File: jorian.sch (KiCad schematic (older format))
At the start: 101 parts, among them J1 USB-C, J2 USB-C, J3 MicroUSB, J4 MicroUSB, J5 MJ-4PP-9, Q1 AO3407, SW1 MSK-12C02, U1 E73-2G4M08S1C-52840, U2 E73-2G4M08S1C-52840, U3 MCP73831, X1 10uH

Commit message: updated files
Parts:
- removed H1: Battery Pad, kbd:battery_pad, symbol Mechanical:MountingHole_Pad
- removed JP1: +, kbd:jumper, symbol Device:Jumper_NO_Small
- removed JP10: -, kbd:jumper, symbol Device:Jumper_NO_Small
- removed JP16, JP25, JP26, JP27, JP28, JP29, JP30, JP31: (no value), kbd:jumper, symbol Device:Jumper_NO_Small
- removed OLED2: I2C_conn, kbd:connector_i2c, symbol Connector_Generic:Conn_01x04
- added Q2: SI2306, Package_TO_SOT_SMD:SOT-23, symbol Transistor_FET:BS870
- added R3: 10K, Resistor_SMD:R_0603_1608Metric, symbol Device:R
- JP11: symbol Connector_Generic:Conn_01x04 -> Connector_Generic:Conn_01x02
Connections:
- net labels added: LED_GND
- net labels removed: PGND
- wire segments 334 -> 317
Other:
- note added: "Power Control\nNormally On\nLow - Off\n"
- moved on the sheet: J5, U1, U2, X1

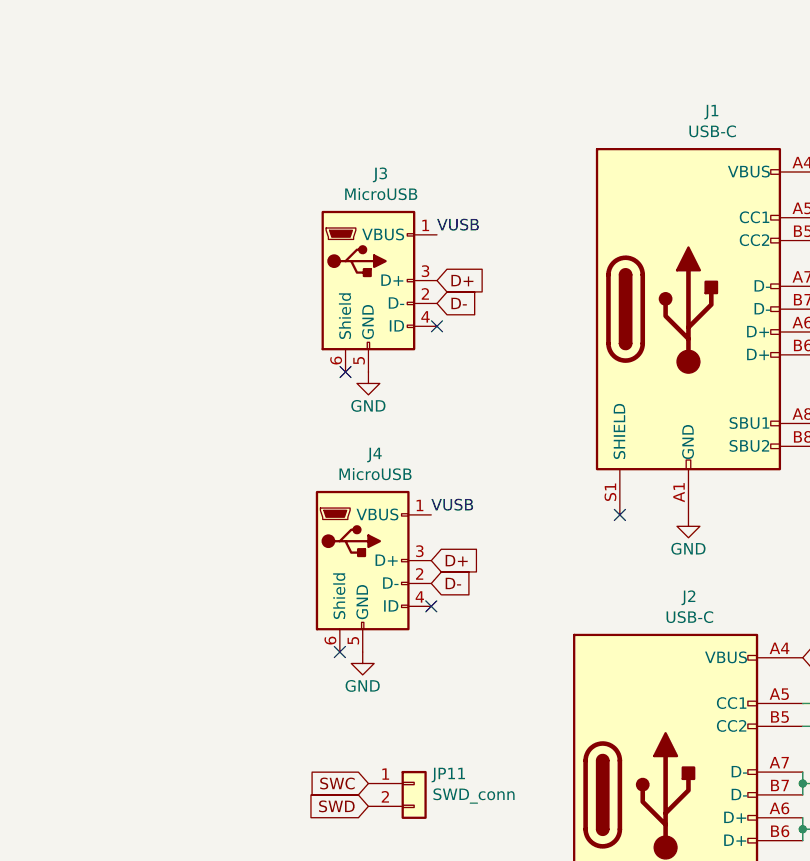
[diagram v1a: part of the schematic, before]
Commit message: updated files
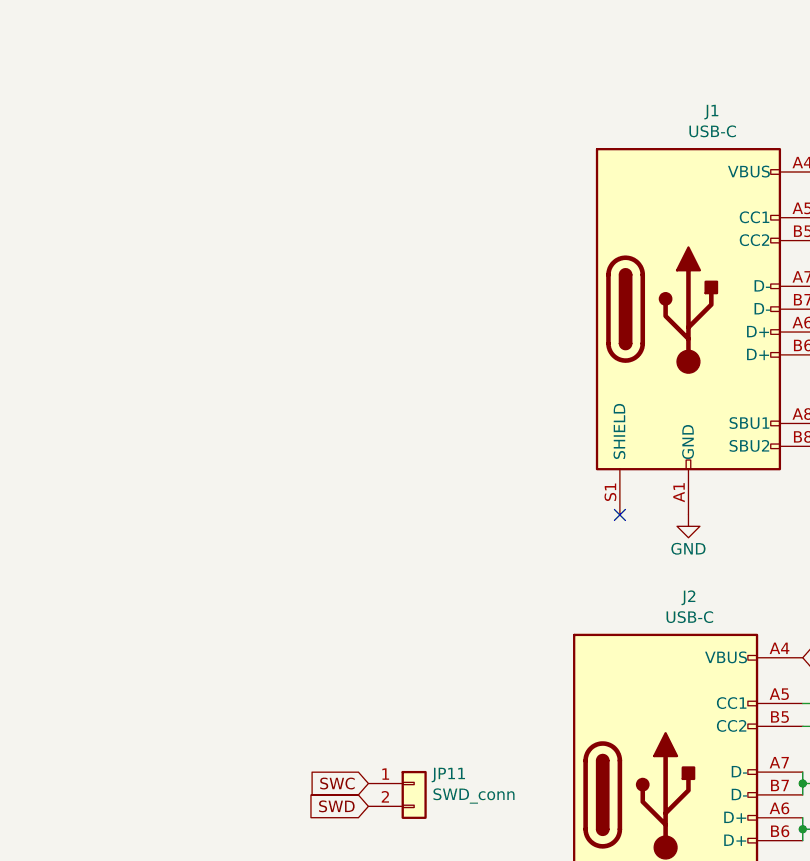
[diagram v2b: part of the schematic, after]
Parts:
- removed J3, J4: MicroUSB, kbd:usb_micro_custom, symbol Connector:USB_B_Micro
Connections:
- no-connect marks 18 -> 14
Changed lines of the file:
@@
 	8000 9300 8500 9300
-$Comp
-L Connector:USB_B_Micro J3
-U 1 1 5DDAA442
-P 13125 5500
-F 0 "J3" H 13180 5967 50  0000 C CNN
-F 1 "MicroUSB" H 13180 5876 50  0000 C CNN
-F 2 "kbd:usb_micro_custom" H 13275 5450 50  0001 C CNN
-F 3 "~" H 13275 5450 50  0001 C CNN
-	1    13125 5500
-	1    0    0    -1
-$EndComp
-Text Label 13425 5300 0    50   ~ 0
-VUSB
-NoConn ~ 13025 5900
 $Comp
 L power:GND #PWR0108
@@
 Wire Wire Line
 	15125 5525 15125 5575
-NoConn ~ 13000 7125
-NoConn ~ 13400 6925
 NoConn ~ 14225 6525
 NoConn ~ 15125 6225
@@
 NoConn ~ 15125 5325
 NoConn ~ 15125 5225
-Text Label 13400 6525 0    50   ~ 0
-VUSB
-$Comp
-L Connector:USB_B_Micro J4
-U 1 1 5DDAA45A
-P 13100 6725
-F 0 "J4" H 13155 7192 50  0000 C CNN
-F 1 "MicroUSB" H 13155 7101 50  0000 C CNN
-F 2 "kbd:usb_micro_custom" H 13250 6675 50  0001 C CNN
-F 3 "~" H 13250 6675 50  0001 C CNN
-	1    13100 6725
-	1    0    0    -1
-$EndComp
 $Comp
 L jorian-rescue:USB_C_Receptacle_USB2.0-Connector J1
@@
 	1    0    0    -1
 $EndComp
-NoConn ~ 13425 5700
-$Comp
-L power:GND #PWR0109
-U 1 1 5DDAA46D
-P 13125 5900
-F 0 "#PWR0109" H 13125 5650 50  0001 C CNN
-F 1 "GND" H 13125 5750 50  0000 C CNN
-F 2 "" H 13125 5900 50  0001 C CNN
-F 3 "" H 13125 5900 50  0001 C CNN
-	1    13125 5900
-	-1   0    0    -1
-$EndComp
-$Comp
-L power:GND #PWR0112
-U 1 1 5DDAA473
-P 13100 7125
-F 0 "#PWR0112" H 13100 6875 50  0001 C CNN
-F 1 "GND" H 13100 6975 50  0000 C CNN
-F 2 "" H 13100 7125 50  0001 C CNN
-F 3 "" H 13100 7125 50  0001 C CNN
-	1    13100 7125
-	-1   0    0    -1
-$EndComp
 Text GLabel 15225 5575 2    50   Input ~ 0
 D-
@@
 Wire Wire Line
 	15125 5775 15225 5775
-Text GLabel 13425 5500 2    50   Input ~ 0
-D+
-Text GLabel 13425 5600 2    50   Input ~ 0
-D-
-Text GLabel 13400 6825 2    50   Input ~ 0
-D-
-Text GLabel 13400 6725 2    50   Input ~ 0
-D+
 Text GLabel 15125 5025 2    50   Input ~ 0
 VUSB

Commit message: updated files
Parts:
- removed JP18: LIPO+, kbd:jumper, symbol Device:Jumper_NO_Small
- removed JP19: LIPO-, kbd:jumper, symbol Device:Jumper_NO_Small
- removed JP20: BAT+, kbd:jumper, symbol Device:Jumper_NO_Small
- removed JP21: BAT-, kbd:jumper, symbol Device:Jumper_NO_Small
- added Q3: AO3407, Package_TO_SOT_SMD:SOT-23, symbol Transistor_FET:BSS83P
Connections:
- net labels added: LED_VCC
- net labels removed: LED_GND, LIPO+, LIPO-
- wire segments 317 -> 320
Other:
- moved on the sheet: BT1, C1, C2, C3, D1, D2, JP11, JP2, JP3, JP4, JP5, JP6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

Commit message: updated files
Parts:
- removed J2: USB-C, kbd:usb_type_c, symbol jorian-rescue:USB_C_Receptacle_USB2.0-Connector
- removed U2: E73-2G4M08S1C-52840, kbd:E73-2G4M08S1C-52840, symbol jorian-rescue:E73-2G4M08S1C-52840
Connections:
- net labels added: CC1, CC2
- wire segments 320 -> 303
- no-connect marks 14 -> 8
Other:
- moved on the sheet: R1, R2

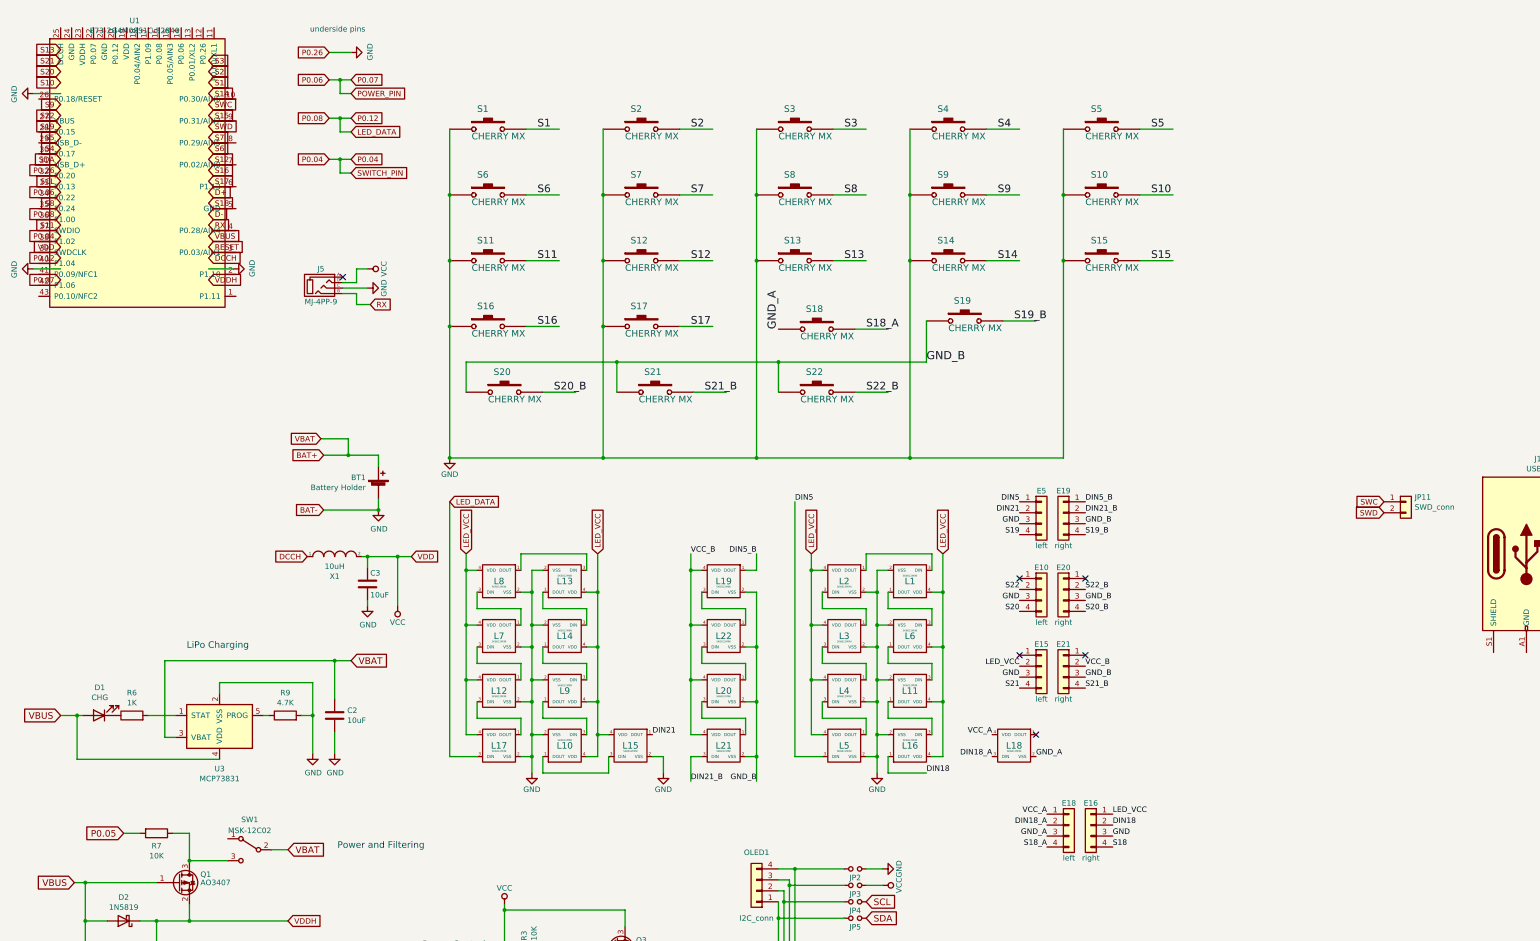
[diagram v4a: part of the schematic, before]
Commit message: autorouted
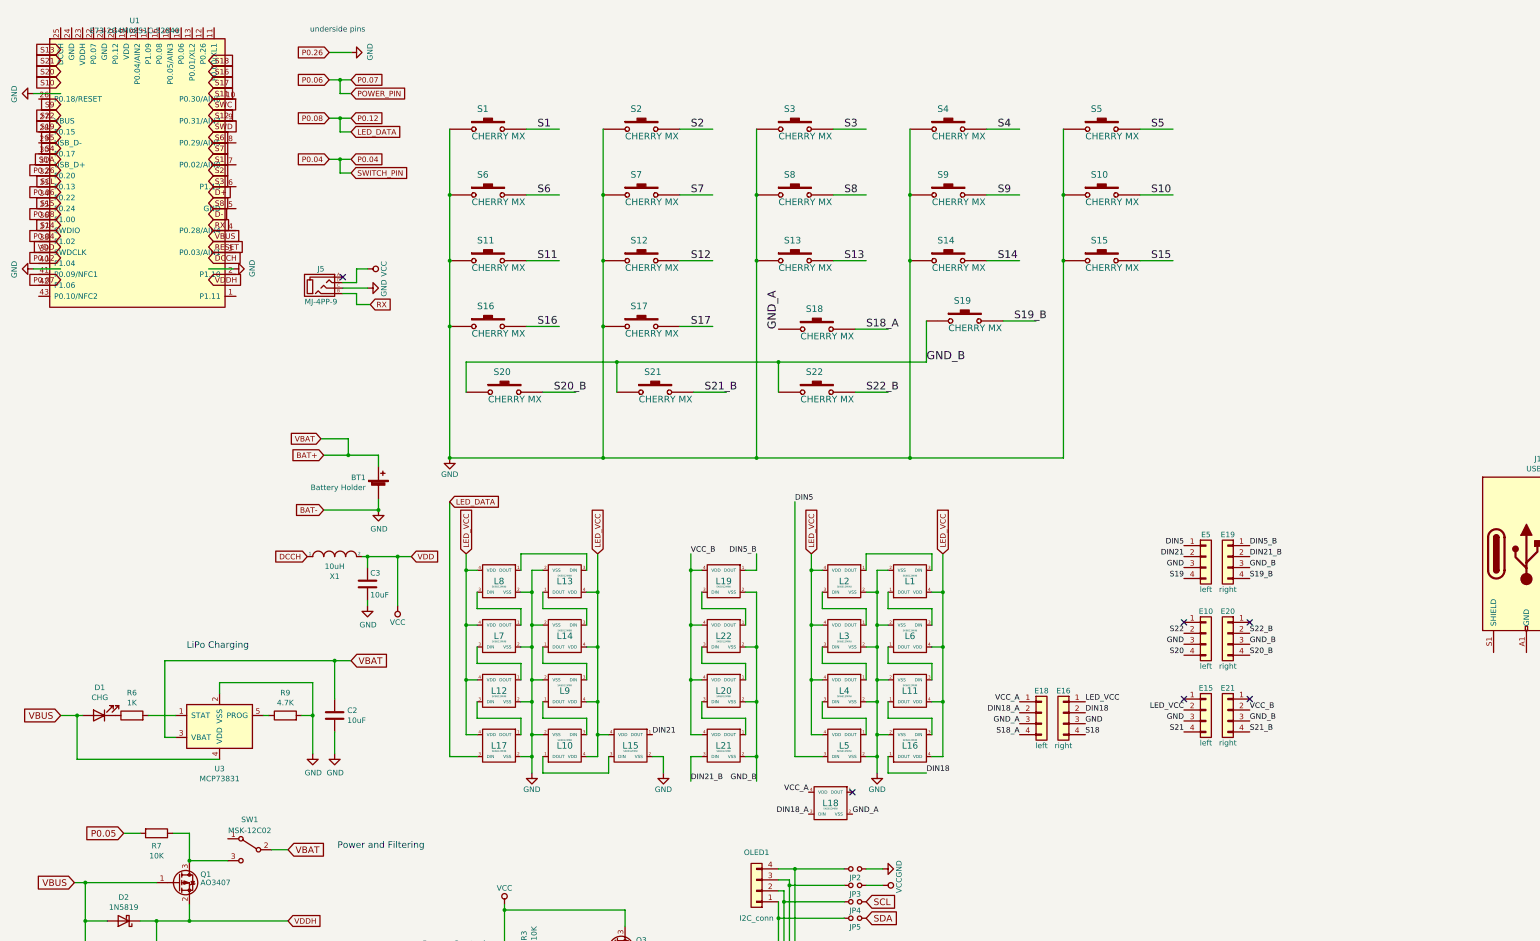
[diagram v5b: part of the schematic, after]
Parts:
- removed JP11: SWD_conn, kbd:connector_swd, symbol Connector_Generic:Conn_01x02
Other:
- moved on the sheet: E10, E15, E16, E18, E19, E20, E21, E5, L18
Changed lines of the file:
@@
 L Connector_Generic:Conn_01x04 E16
 U 1 1 5C28A7CD
-P 10550 8100
-F 0 "E16" H 10550 8300 50  0000 C CNN
-F 1 "right" H 10550 7800 50  0000 C CNN
-F 2 "kbd:edge_conn" H 10550 8100 50  0001 C CNN
-F 3 "" H 10550 8100 50  0001 C CNN
-	1    10550 8100
+P 10300 7075
+F 0 "E16" H 10300 7275 50  0000 C CNN
+F 1 "right" H 10300 6775 50  0000 C CNN
+F 2 "kbd:edge_conn" H 10300 7075 50  0001 C CNN
+F 3 "" H 10300 7075 50  0001 C CNN
+	1    10300 7075
 	-1   0    0    -1
 $EndComp
@@
 L Connector_Generic:Conn_01x04 E18
 U 1 1 5C28AA80
-P 10350 8100
-F 0 "E18" H 10350 8300 50  0000 C CNN
-F 1 "left" H 10350 7800 50  0000 C CNN
-F 2 "kbd:edge_conn" H 10350 8100 50  0001 C CNN
-F 3 "" H 10350 8100 50  0001 C CNN
-	1    10350 8100
-	1    0    0    -1
-$EndComp
-Text Label 10750 8200 0    50   ~ 0
+P 10100 7075
+F 0 "E18" H 10100 7275 50  0000 C CNN
+F 1 "left" H 10100 6775 50  0000 C CNN
+F 2 "kbd:edge_conn" H 10100 7075 50  0001 C CNN
+F 3 "" H 10100 7075 50  0001 C CNN
+	1    10100 7075
+	1    0    0    -1
+$EndComp
+Text Label 10500 7175 0    50   ~ 0
 GND
-Text Label 10750 8300 0    50   ~ 0
+Text Label 10500 7275 0    50   ~ 0
 S18
-Text Label 10750 8000 0    50   ~ 0
+Text Label 10500 6975 0    50   ~ 0
 LED_VCC
 $Comp
 L Connector_Generic:Conn_01x04 E19
 U 1 1 5C6E087C
-P 10300 5250
-F 0 "E19" H 10300 5450 50  0000 C CNN
-F 1 "right" H 10300 4950 50  0000 C CNN
-F 2 "kbd:edge_conn" H 10300 5250 50  0001 C CNN
-F 3 "" H 10300 5250 50  0001 C CNN
-	1    10300 5250
+P 11800 5650
+F 0 "E19" H 11800 5850 50  0000 C CNN
+F 1 "right" H 11800 5350 50  0000 C CNN
+F 2 "kbd:edge_conn" H 11800 5650 50  0001 C CNN
+F 3 "" H 11800 5650 50  0001 C CNN
+	1    11800 5650
 	-1   0    0    -1
 $EndComp
@@
 L Connector_Generic:Conn_01x04 E5
 U 1 1 5C6E0883
-P 10100 5250
-F 0 "E5" H 10100 5450 50  0000 C CNN
-F 1 "left" H 10100 4950 50  0000 C CNN
-F 2 "kbd:edge_conn" H 10100 5250 50  0001 C CNN
-F 3 "" H 10100 5250 50  0001 C CNN
-	1    10100 5250
-	1    0    0    -1
-$EndComp
-Text Label 9900 5450 2    50   ~ 0
+P 11600 5650
+F 0 "E5" H 11600 5850 50  0000 C CNN
+F 1 "left" H 11600 5350 50  0000 C CNN
+F 2 "kbd:edge_conn" H 11600 5650 50  0001 C CNN
+F 3 "" H 11600 5650 50  0001 C CNN
+	1    11600 5650
+	1    0    0    -1
+$EndComp
+Text Label 11400 5850 2    50   ~ 0
 S19
-Text Label 9900 6150 2    50   ~ 0
+Text Label 11400 6550 2    50   ~ 0
 S20
 $Comp
 L Connector_Generic:Conn_01x04 E21
 U 1 1 5C6F2906
-P 10300 6650
-F 0 "E21" H 10300 6850 50  0000 C CNN
-F 1 "right" H 10300 6350 50  0000 C CNN
-F 2 "kbd:edge_conn" H 10300 6650 50  0001 C CNN
-F 3 "" H 10300 6650 50  0001 C CNN
-	1    10300 6650
+P 11800 7050
+F 0 "E21" H 11800 7250 50  0000 C CNN
+F 1 "right" H 11800 6750 50  0000 C CNN
+F 2 "kbd:edge_conn" H 11800 7050 50  0001 C CNN
+F 3 "" H 11800 7050 50  0001 C CNN
+	1    11800 7050
 	-1   0    0    -1
 $EndComp
@@
 L Connector_Generic:Conn_01x04 E15
 U 1 1 5C6F290D
-P 10100 6650
-F 0 "E15" H 10100 6850 50  0000 C CNN
-F 1 "left" H 10100 6350 50  0000 C CNN
-F 2 "kbd:edge_conn" H 10100 6650 50  0001 C CNN
-F 3 "" H 10100 6650 50  0001 C CNN
-	1    10100 6650
-	1    0    0    -1
-$EndComp
-Text Label 9900 5950 2    50   ~ 0
+P 11600 7050
+F 0 "E15" H 11600 7250 50  0000 C CNN
+F 1 "left" H 11600 6750 50  0000 C CNN
+F 2 "kbd:edge_conn" H 11600 7050 50  0001 C CNN
+F 3 "" H 11600 7050 50  0001 C CNN
+	1    11600 7050
+	1    0    0    -1
+$EndComp
+Text Label 11400 6350 2    50   ~ 0
 S22
-Text Label 10750 8100 0    50   ~ 0
+Text Label 10500 7075 0    50   ~ 0
 DIN18
-Text Label 10150 8300 2    50   ~ 0
+Text Label 9900 7275 2    50   ~ 0
 S18_A
-Text Label 10150 8200 2    50   ~ 0
+Text Label 9900 7175 2    50   ~ 0
 GND_A
-Text Label 10150 8000 2    50   ~ 0
+Text Label 9900 6975 2    50   ~ 0
 VCC_A
-Text Label 10150 8100 2    50   ~ 0
+Text Label 9900 7075 2    50   ~ 0
 DIN18_A
-Text Label 10500 5450 0    50   ~ 0
+Text Label 12000 5850 0    50   ~ 0
 S19_B
-Text Label 10500 6150 0    50   ~ 0
+Text Label 12000 6550 0    50   ~ 0
 S20_B
-Text Label 10500 6850 0    50   ~ 0
+Text Label 12000 7250 0    50   ~ 0
 S21_B
-Text Label 10500 5950 0    50   ~ 0
+Text Label 12000 6350 0    50   ~ 0
 S22_B
-Text Label 10500 6650 0    50   ~ 0
+Text Label 12000 7050 0    50   ~ 0
 VCC_B
-Text Label 10500 5250 0    50   ~ 0
+Text Label 12000 5650 0    50   ~ 0
 DIN21_B
-Text Label 9900 5150 2    50   ~ 0
+Text Label 11400 5550 2    50   ~ 0
 DIN5
-Text Label 10500 5150 0    50   ~ 0
+Text Label 12000 5550 0    50   ~ 0
 DIN5_B
-Text Label 9900 5250 2    50   ~ 0
+Text Label 11400 5650 2    50   ~ 0
 DIN21
 $Comp
@@
 L Connector_Generic:Conn_01x04 E20
 U 1 1 5C1C4E7E
-P 10300 5950
-F 0 "E20" H 10300 6150 50  0000 C CNN
-F 1 "right" H 10300 5650 50  0000 C CNN
-F 2 "kbd:edge_conn" H 10300 5950 50  0001 C CNN
-F 3 "" H 10300 5950 50  0001 C CNN
-	1    10300 5950
+P 11800 6350
+F 0 "E20" H 11800 6550 50  0000 C CNN
+F 1 "right" H 11800 6050 50  0000 C CNN
+F 2 "kbd:edge_conn" H 11800 6350 50  0001 C CNN
+F 3 "" H 11800 6350 50  0001 C CNN
+	1    11800 6350
 	-1   0    0    -1
 $EndComp
@@
 L Connector_Generic:Conn_01x04 E10
 U 1 1 5C1C4E85
-P 10100 5950
-F 0 "E10" H 10100 6150 50  0000 C CNN
-F 1 "left" H 10100 5650 50  0000 C CNN
-F 2 "kbd:edge_conn" H 10100 5950 50  0001 C CNN
-F 3 "" H 10100 5950 50  0001 C CNN
-	1    10100 5950
+P 11600 6350
+F 0 "E10" H 11600 6550 50  0000 C CNN
+F 1 "left" H 11600 6050 50  0000 C CNN
+F 2 "kbd:edge_conn" H 11600 6350 50  0001 C CNN
+F 3 "" H 11600 6350 50  0001 C CNN
+	1    11600 6350
 	1    0    0    -1
 $EndComp
@@
 L kbd:kbd_SK6812MINI L18
 U 1 1 5C54BB48
-P 9850 7375
-F 0 "L18" H 9850 7375 59  0000 C CNN
-F 1 "SK6812MINI" H 9850 7325 16  0000 C CNN
-F 2 "kbd:kbd_SK6812MINI" H 9850 7375 60  0001 C CNN
-F 3 "" H 9850 7375 60  0001 C CNN
-	1    9850 7375
+P 8175 7900
+F 0 "L18" H 8175 7900 59  0000 C CNN
+F 1 "SK6812MINI" H 8175 7850 16  0000 C CNN
+F 2 "kbd:kbd_SK6812MINI" H 8175 7900 60  0001 C CNN
+F 3 "" H 8175 7900 60  0001 C CNN
+	1    8175 7900
 	-1   0    0    -1
 $EndComp
-Text Label 9650 7275 2    50   ~ 0
+Text Label 7975 7800 2    50   ~ 0
 VCC_A
-Text Label 9650 7475 2    50   ~ 0
+Text Label 7975 8000 2    50   ~ 0
 DIN18_A
-Text Label 10050 7475 0    50   ~ 0
+Text Label 8375 8000 0    50   ~ 0
 GND_A
-NoConn ~ 10050 7275
+NoConn ~ 8375 7800
 Wire Wire Line
 	6100 3550 6100 4750
@@
 	0    -1   -1   0
 $EndComp
-Text GLabel 2500 1325 2    50   Input ~ 0
+Text GLabel 2500 2025 2    50   Input ~ 0
 S1
 $Comp
@@
 	1    0    0    -1
 $EndComp
-Text GLabel 2500 1225 2    50   Input ~ 0
+Text GLabel 2500 2125 2    50   Input ~ 0
 S2
-Text GLabel 2500 1125 2    50   Input ~ 0
+Text GLabel 2500 2225 2    50   Input ~ 0
 S3
 Text GLabel 1150 1925 0    50   Input ~ 0
@@
 Text GLabel 1150 1825 0    50   Input ~ 0
 S5
+Text GLabel 2500 1825 2    50   Input ~ 0
+S6
 Text GLabel 2500 1925 2    50   Input ~ 0
-S6
-Text GLabel 2500 1825 2    50   Input ~ 0
 S7
-Text GLabel 1150 2425 0    50   Input ~ 0
+Text GLabel 2500 2425 2    50   Input ~ 0
 S8
 Text GLabel 1150 1525 0    50   Input ~ 0
@@
 Text GLabel 1150 1325 0    50   Input ~ 0
 S10
-Text GLabel 1150 2625 0    50   Input ~ 0
+Text GLabel 2500 1425 2    50   Input ~ 0
 S11
-Text GLabel 2500 2025 2    50   Input ~ 0
+Text GLabel 2500 1625 2    50   Input ~ 0
 S12
 Text GLabel 1150 1025 0    50   Input ~ 0
 S13
-Text GLabel 2500 1425 2    50   Input ~ 0
+Text GLabel 1150 2625 0    50   Input ~ 0
 S14
-Text GLabel 2500 1625 2    50   Input ~ 0
+Text GLabel 1150 2425 0    50   Input ~ 0
 S15
-Text GLabel 2500 2125 2    50   Input ~ 0
+Text GLabel 2500 1225 2    50   Input ~ 0
 S16
-Text GLabel 2500 2225 2    50   Input ~ 0
+Text GLabel 2500 1325 2    50   Input ~ 0
 S17
-Text GLabel 2500 2425 2    50   Input ~ 0
+Text GLabel 2500 1125 2    50   Input ~ 0
 S18
 Text GLabel 1150 1725 0    50   Input ~ 0
@@
 Text GLabel 2500 2625 2    50   Input ~ 0
 RX
-Text Label 9900 6750 2    50   ~ 0
+Text Label 11400 7150 2    50   ~ 0
 GND
-Text Label 10500 6750 0    50   ~ 0
+Text Label 12000 7150 0    50   ~ 0
 GND_B
-Text Label 9900 6050 2    50   ~ 0
+Text Label 11400 6450 2    50   ~ 0
 GND
-Text Label 9900 6650 2    50   ~ 0
+Text Label 11400 7050 2    50   ~ 0
 LED_VCC
-Text Label 9900 6850 2    50   ~ 0
+Text Label 11400 7250 2    50   ~ 0
 S21
-Text Label 9900 5350 2    50   ~ 0
+Text Label 11400 5750 2    50   ~ 0
 GND
-Text Label 10500 5350 0    50   ~ 0
+Text Label 12000 5750 0    50   ~ 0
 GND_B
-NoConn ~ 10500 6550
-NoConn ~ 9900 6550
-NoConn ~ 9900 5850
-NoConn ~ 10500 5850
-Text Label 10500 6050 0    50   ~ 0
+NoConn ~ 12000 6950
+NoConn ~ 11400 6950
+NoConn ~ 11400 6250
+NoConn ~ 12000 6250
+Text Label 12000 6450 0    50   ~ 0
 GND_B
-Text GLabel 13225 5150 0    50   Input ~ 0
-SWC
-Text GLabel 13225 5250 0    50   Input ~ 0
-SWD
-$Comp
-L Connector_Generic:Conn_01x02 JP11
-U 1 1 5DDAA467
-P 13425 5150
-F 0 "JP11" H 13505 5192 50  0000 L CNN
-F 1 "SWD_conn" H 13505 5101 50  0000 L CNN
-F 2 "kbd:connector_swd" H 13425 5150 50  0001 C CNN
-F 3 "~" H 13425 5150 50  0001 C CNN
-	1    13425 5150
-	1    0    0    -1
-$EndComp
 $Comp
 L Transistor_FET:BS870 Q2
